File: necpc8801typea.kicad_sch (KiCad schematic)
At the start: 258 parts, among them J2 Conn_01x04_MountingPin, Q1 Q_PMOS_GSD AO3401A, Q2 Q_NMOS_GSD 2N7002, Q3 Q_NMOS_GSD 2N7002, Q4 2N3904, SW1 SW_Push, U1 XC6206P332NR, U2 74AHCT1G125, U3 STM32F401RETx, U4 24LC64, U5 USBLC6-2SC6, Y1 8MHz

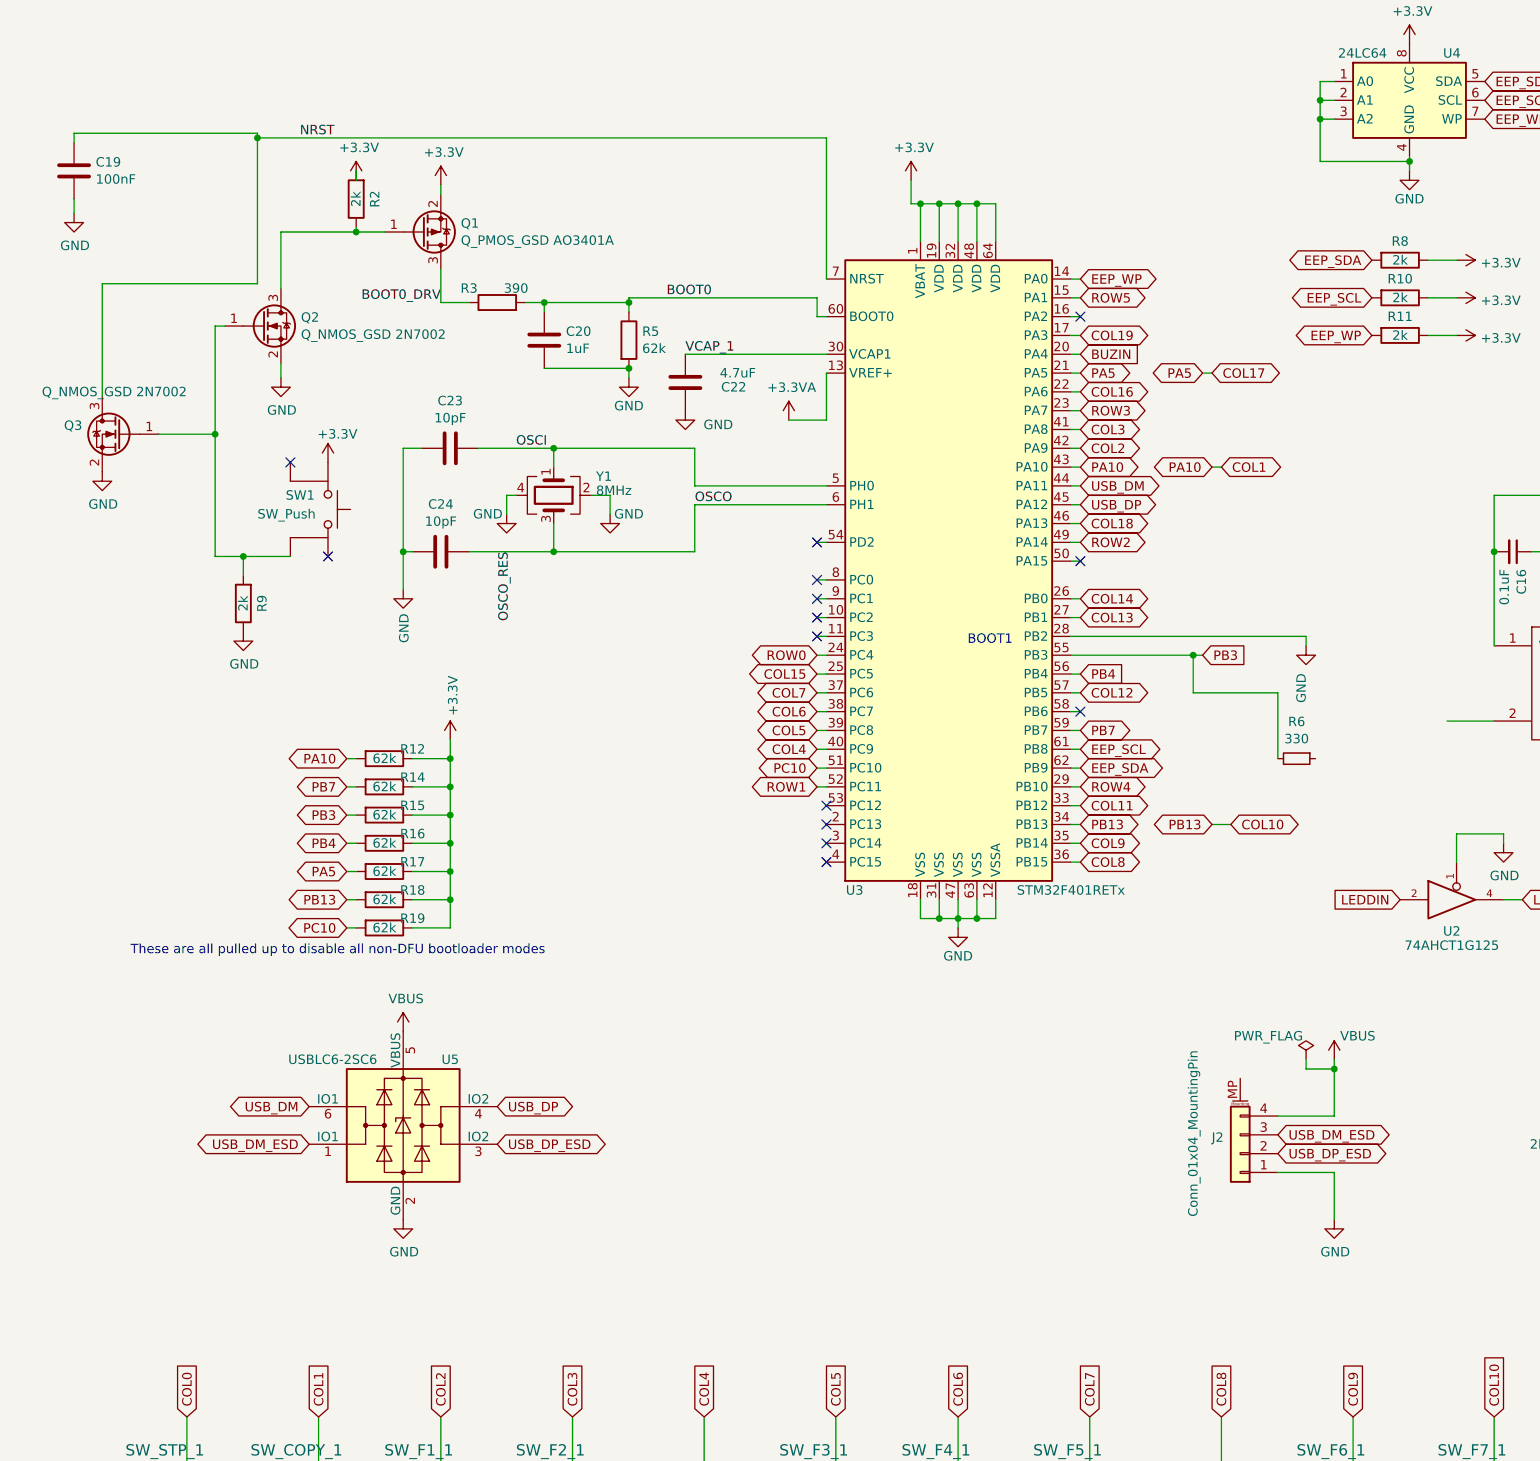
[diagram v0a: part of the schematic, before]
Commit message: fixes
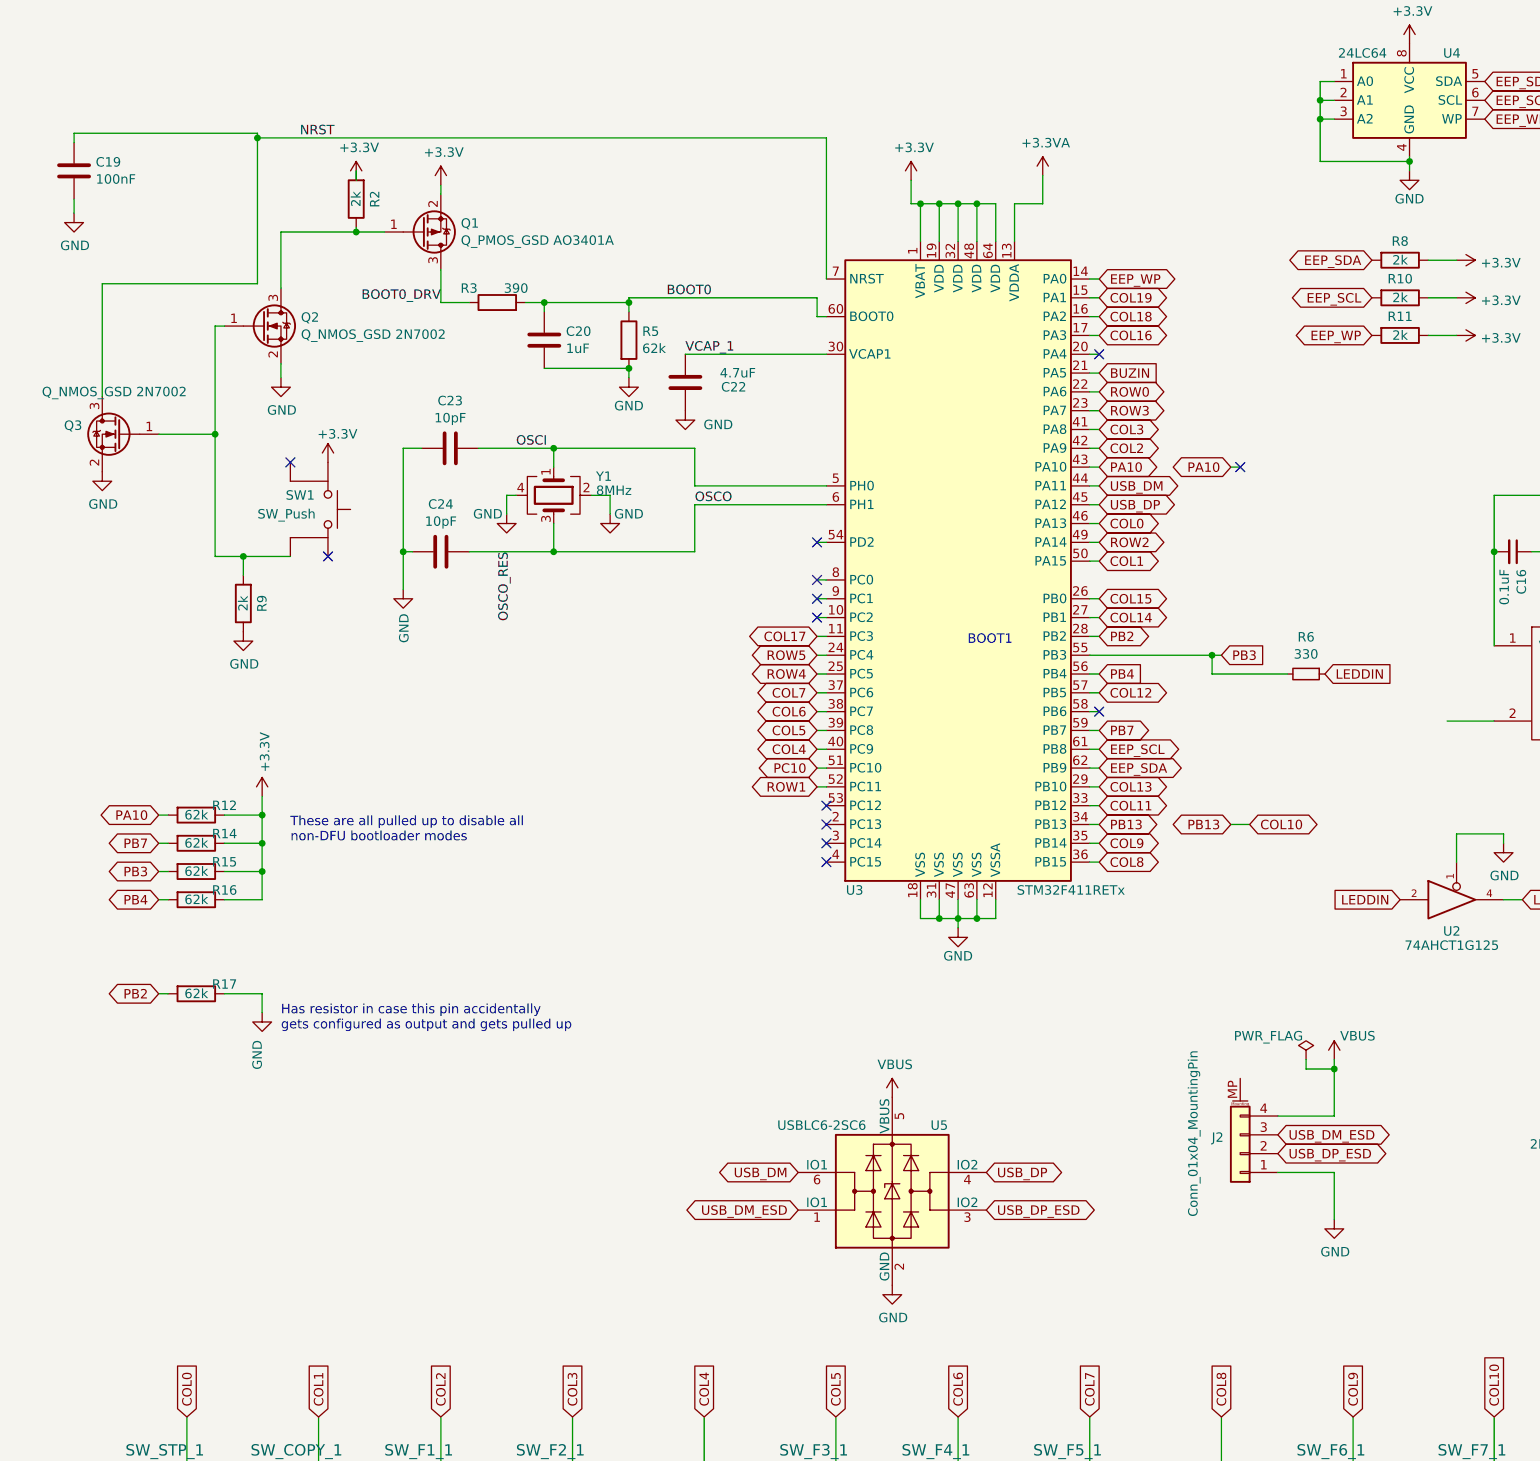
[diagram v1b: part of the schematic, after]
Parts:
- removed R18, R19: 62k, Resistor_SMD:R_0805_2012Metric_Pad1.20x1.40mm_HandSolder, symbol Device:R
- U3: value STM32F401RETx -> STM32F411RETx; symbol MCU_ST_STM32F4:STM32F401RETx -> MCU_ST_STM32F4:STM32F411RETx
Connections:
- net +3.3VA: no longer R17.1
- net BUZIN: now also U3.21 (PA5); no longer U3.20 (PA4)
- net COL0: now also U3.46 (PA13)
- net COL1: now also U3.50 (PA15); no longer R12.2, U3.43 (PA10)
- net COL13: now also U3.29 (PB10); no longer U3.27 (PB1)
- net COL14: now also U3.27 (PB1); no longer U3.26 (PB0)
- net COL15: now also U3.26 (PB0); no longer U3.25 (PC5)
- net COL16: now also U3.17 (PA3); no longer U3.22 (PA6)
- net COL17: now also U3.11 (PC3); no longer R17.2, U3.21 (PA5)
- net COL18: now also U3.16 (PA2); no longer U3.46 (PA13)
- net COL19: now also U3.15 (PA1); no longer U3.17 (PA3)
- net GND: now also R17.1; no longer U3.28 (PB2)
- net LEDDIN: now also R6.1
- net ROW0: now also U3.22 (PA6); no longer U3.24 (PC4)
- net ROW4: now also U3.25 (PC5); no longer U3.29 (PB10)
- net ROW5: now also U3.24 (PC4); no longer U3.15 (PA1)
- new net PA10: R12.2, U3.43 (PA10)
- new net PB2: R17.2, U3.28 (PB2)
- no-connect marks 14 -> 13
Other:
- note added: "Has resistor in case this pin accidentally gets configured as output and gets pulled up"
- moved on the sheet: R12, R14, R15, R16, R17, R6, U3

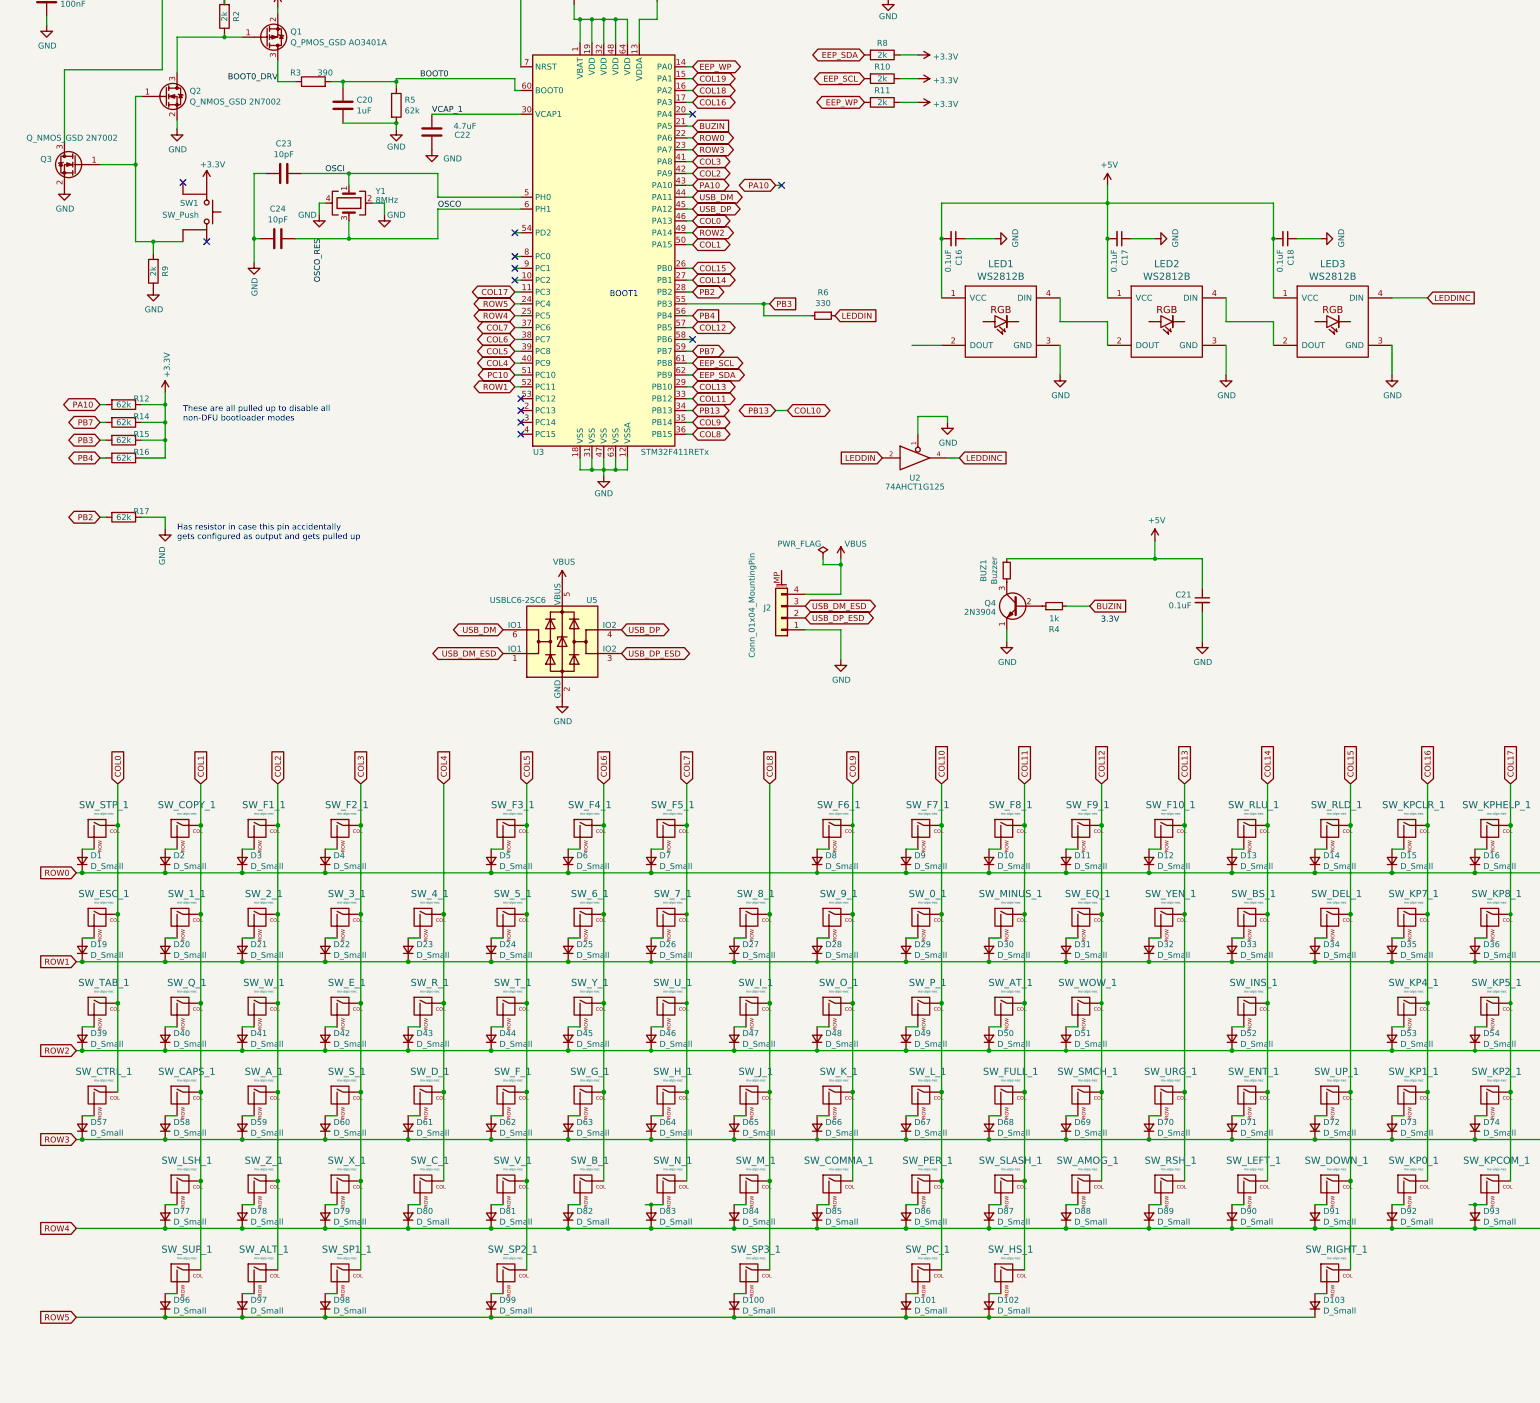
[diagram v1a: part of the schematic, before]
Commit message: fixes
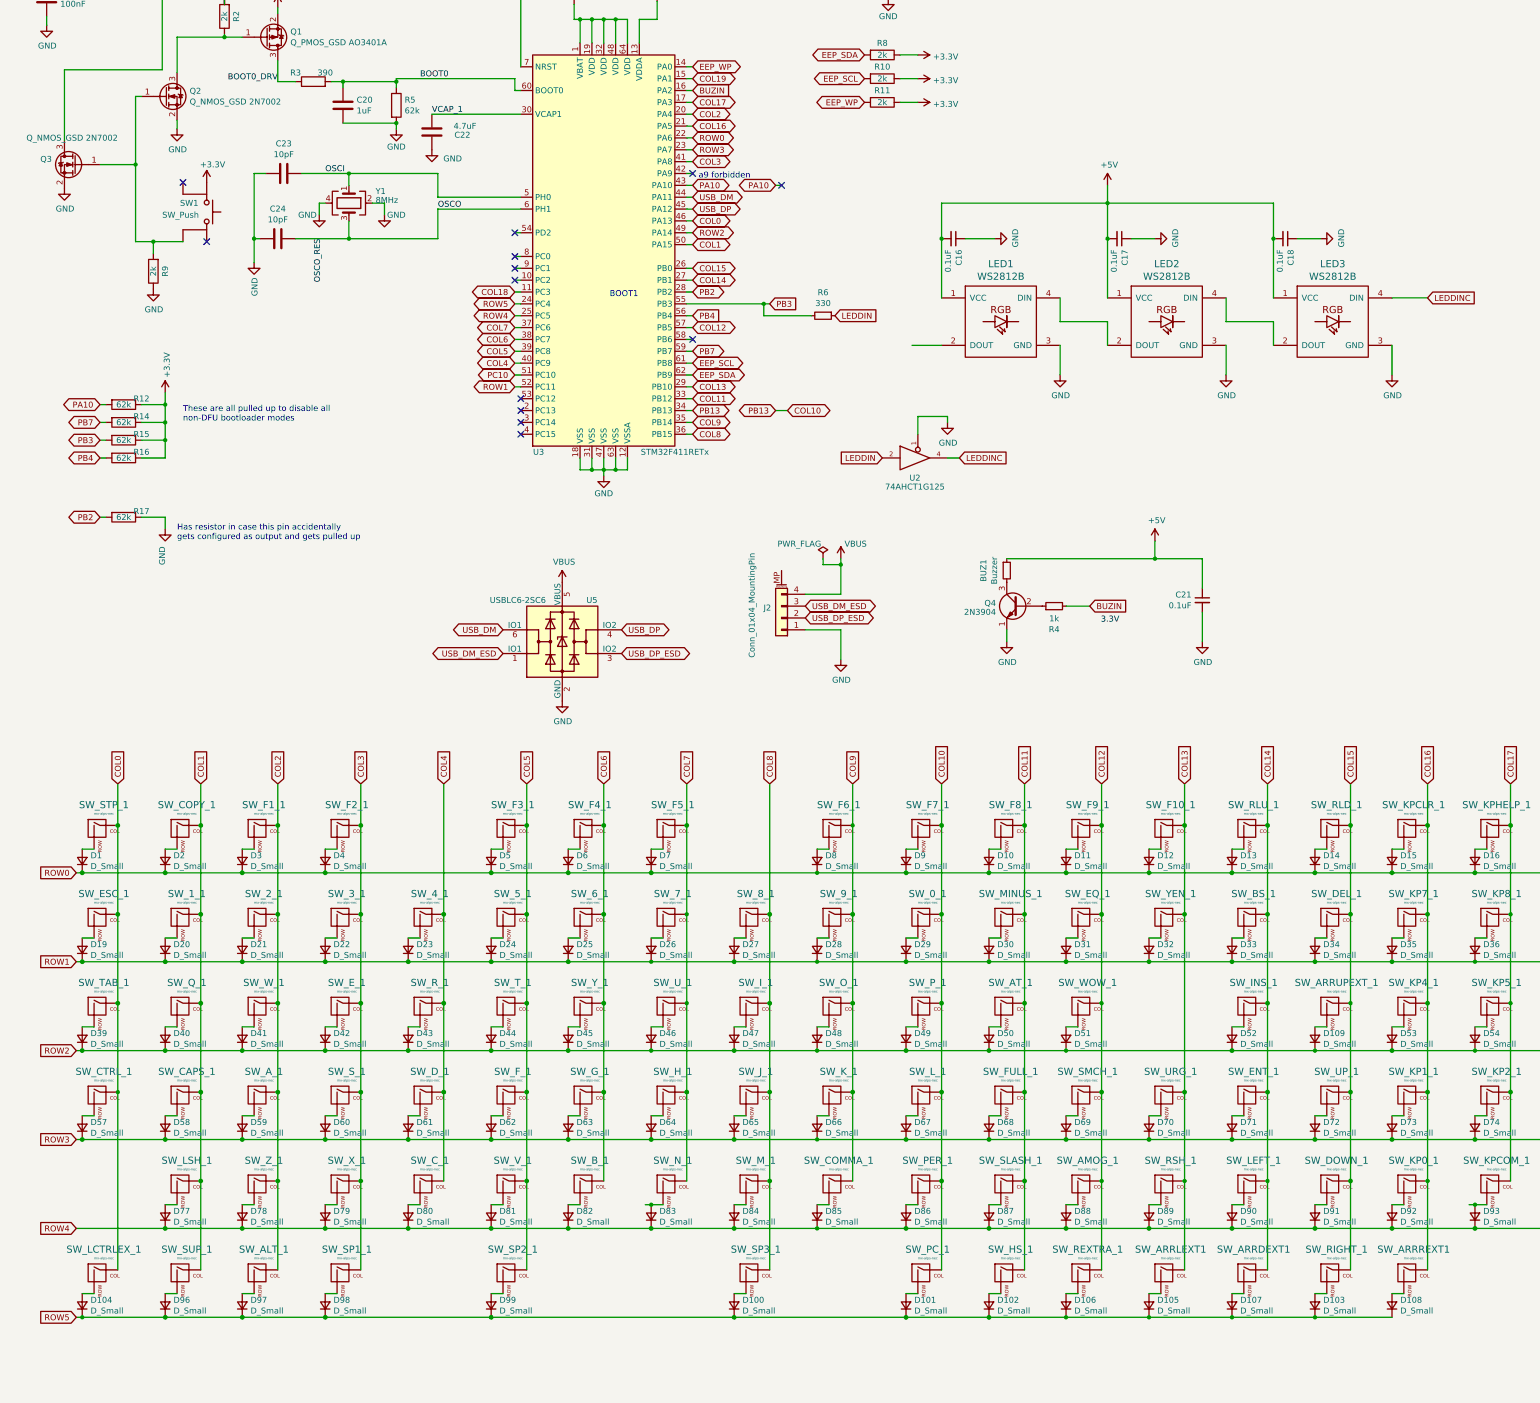
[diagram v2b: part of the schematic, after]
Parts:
- added D104, D105, D106, D107, D108, D109: D_Small, Diode_SMD:D_SOD-123, symbol Device:D_Small
- added SW_ARRDEXT1, SW_ARRLEXT1, SW_ARRREXT1, SW_ARRUPEXT_1, SW_LCTRLEX_1, SW_REXTRA_1: mx-alps-nec, MX_NEC:mx-nec-alps, symbol MX_Alps_Hybrid:mx-alps-nec
- SW1: footprint random-keyboard-parts:SKQG-1155865 -> controller:switch_K2-1187SQ-A4SW-06
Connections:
- net BUZIN: now also U3.16 (PA2); no longer U3.21 (PA5)
- net COL0: now also SW_LCTRLEX_1.1 (COL)
- net COL12: now also SW_REXTRA_1.1 (COL)
- net COL13: now also SW_ARRLEXT1.1 (COL)
- net COL14: now also SW_ARRDEXT1.1 (COL)
- net COL15: now also SW_ARRUPEXT_1.1 (COL)
- net COL16: now also U3.21 (PA5), SW_ARRREXT1.1 (COL); no longer U3.17 (PA3)
- net COL17: now also U3.17 (PA3); no longer U3.11 (PC3)
- net COL18: now also U3.11 (PC3); no longer U3.16 (PA2)
- net COL2: now also U3.20 (PA4); no longer U3.42 (PA9)
- net ROW2: now also D109.1 (K)
- net ROW5: now also D104.1 (K), D105.1 (K), D106.1 (K), D107.1 (K), D108.1 (K)
- new net: D106.2 (A), SW_REXTRA_1.2 (ROW)
- new net: D108.2 (A), SW_ARRREXT1.2 (ROW)
- new net: D104.2 (A), SW_LCTRLEX_1.2 (ROW)
- new net: D105.2 (A), SW_ARRLEXT1.2 (ROW)
- new net: D109.2 (A), SW_ARRUPEXT_1.2 (ROW)
- new net: D107.2 (A), SW_ARRDEXT1.2 (ROW)
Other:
- note added: "a9 forbidden"
